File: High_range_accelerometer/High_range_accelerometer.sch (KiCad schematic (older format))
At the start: 55 parts, among them J1 USB_B_Micro, P1 KRC_PSoCWriter, U1 KRC_Conn_CAN, U2 NCP718ASN330T1G, U3 NCP718ASN500T1G, U4 NCV7342, U5 CY8C5868LTI-LP039, U6 H3LIS331DLTR, U7 W25N01GVxxIG-IT, Y2 Crystal_MHz

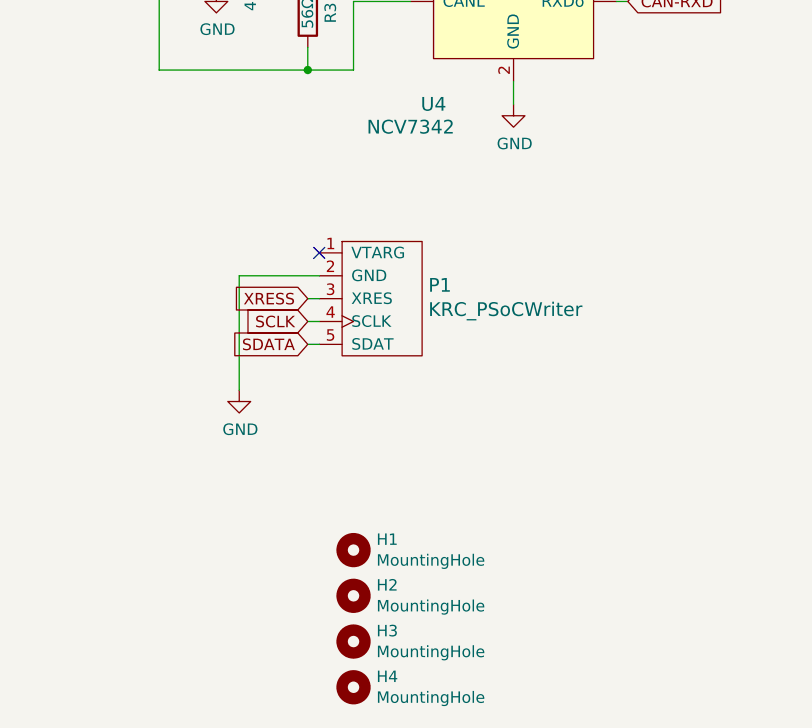
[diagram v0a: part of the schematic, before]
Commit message: add SVG and PDF and Gerber files
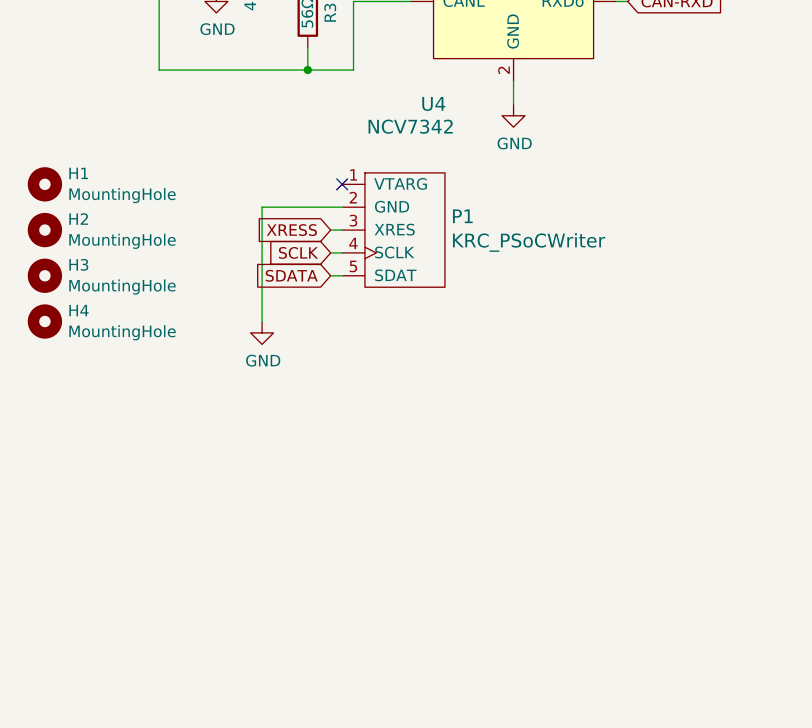
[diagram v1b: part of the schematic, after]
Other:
- moved on the sheet: H1, H2, H3, H4, P1
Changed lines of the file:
@@
 L High_range_accelerometer-rescue:KRC_PSoCWriter-KUT_Connector P1
 U 1 1 5D89CA7D
-P 2100 5500
-F 0 "P1" H 2377 5558 60  0000 L CNN
-F 1 "KRC_PSoCWriter" H 2377 5452 60  0000 L CNN
-F 2 "KUTKiCad_footprint:JST_JQ_05JQ-BT_1x05_P2.5mm_Vertical" H 2325 5500 60  0001 C CNN
-F 3 "" H 2325 5500 60  0000 C CNN
-	1    2100 5500
+P 2200 5200
+F 0 "P1" H 2477 5258 60  0000 L CNN
+F 1 "KRC_PSoCWriter" H 2477 5152 60  0000 L CNN
+F 2 "KUTKiCad_footprint:JST_JQ_05JQ-BT_1x05_P2.5mm_Vertical" H 2425 5200 60  0001 C CNN
+F 3 "" H 2425 5200 60  0000 C CNN
+	1    2200 5200
 	1    0    0    -1
 $EndComp
@@
 L power:GND #PWR03
 U 1 1 5D8A2416
-P 1550 5900
-F 0 "#PWR03" H 1550 5650 50  0001 C CNN
-F 1 "GND" H 1555 5727 50  0000 C CNN
-F 2 "" H 1550 5900 50  0001 C CNN
-F 3 "" H 1550 5900 50  0001 C CNN
-	1    1550 5900
-	1    0    0    -1
-$EndComp
-Wire Wire Line
-	1550 5900 1550 5400
-Wire Wire Line
-	1550 5400 1900 5400
-Text GLabel 1850 5500 0    50   Input ~ 0
+P 1650 5600
+F 0 "#PWR03" H 1650 5350 50  0001 C CNN
+F 1 "GND" H 1655 5427 50  0000 C CNN
+F 2 "" H 1650 5600 50  0001 C CNN
+F 3 "" H 1650 5600 50  0001 C CNN
+	1    1650 5600
+	1    0    0    -1
+$EndComp
+Wire Wire Line
+	1650 5600 1650 5100
+Wire Wire Line
+	1650 5100 2000 5100
+Text GLabel 1950 5200 0    50   Input ~ 0
 XRESS
-Text GLabel 1850 5600 0    50   Input ~ 0
+Text GLabel 1950 5300 0    50   Input ~ 0
 SCLK
-Text GLabel 1850 5700 0    50   Input ~ 0
+Text GLabel 1950 5400 0    50   Input ~ 0
 SDATA
 Wire Wire Line
-	1850 5700 1900 5700
-Wire Wire Line
-	1900 5600 1850 5600
-Wire Wire Line
-	1850 5500 1900 5500
+	1950 5400 2000 5400
+Wire Wire Line
+	2000 5300 1950 5300
+Wire Wire Line
+	1950 5200 2000 5200
 Text GLabel 4550 4150 0    50   Input ~ 0
 XRESS
@@
 Wire Wire Line
 	3250 4200 3200 4200
-NoConn ~ 1900 5300
+NoConn ~ 2000 5000
 $Comp
 L Device:Crystal Y2
@@
 L Mechanical:MountingHole H1
 U 1 1 5D9A09FB
-P 2050 6600
-F 0 "H1" H 2150 6646 50  0000 L CNN
-F 1 "MountingHole" H 2150 6555 50  0000 L CNN
-F 2 "MountingHole:MountingHole_3.2mm_M3" H 2050 6600 50  0001 C CNN
-F 3 "~" H 2050 6600 50  0001 C CNN
-	1    2050 6600
+P 700 5000
+F 0 "H1" H 800 5046 50  0000 L CNN
+F 1 "MountingHole" H 800 4955 50  0000 L CNN
+F 2 "MountingHole:MountingHole_3.2mm_M3" H 700 5000 50  0001 C CNN
+F 3 "~" H 700 5000 50  0001 C CNN
+	1    700  5000
 	1    0    0    -1
 $EndComp
@@
 L Mechanical:MountingHole H2
 U 1 1 5D9A0A93
-P 2050 6800
-F 0 "H2" H 2150 6846 50  0000 L CNN
-F 1 "MountingHole" H 2150 6755 50  0000 L CNN
-F 2 "MountingHole:MountingHole_3.2mm_M3" H 2050 6800 50  0001 C CNN
-F 3 "~" H 2050 6800 50  0001 C CNN
-	1    2050 6800
+P 700 5200
+F 0 "H2" H 800 5246 50  0000 L CNN
+F 1 "MountingHole" H 800 5155 50  0000 L CNN
+F 2 "MountingHole:MountingHole_3.2mm_M3" H 700 5200 50  0001 C CNN
+F 3 "~" H 700 5200 50  0001 C CNN
+	1    700  5200
 	1    0    0    -1
 $EndComp
@@
 L Mechanical:MountingHole H3
 U 1 1 5D9A0B13
-P 2050 7000
-F 0 "H3" H 2150 7046 50  0000 L CNN
-F 1 "MountingHole" H 2150 6955 50  0000 L CNN
-F 2 "MountingHole:MountingHole_3.2mm_M3" H 2050 7000 50  0001 C CNN
-F 3 "~" H 2050 7000 50  0001 C CNN
-	1    2050 7000
+P 700 5400
+F 0 "H3" H 800 5446 50  0000 L CNN
+F 1 "MountingHole" H 800 5355 50  0000 L CNN
+F 2 "MountingHole:MountingHole_3.2mm_M3" H 700 5400 50  0001 C CNN
+F 3 "~" H 700 5400 50  0001 C CNN
+	1    700  5400
 	1    0    0    -1
 $EndComp
@@
 L Mechanical:MountingHole H4
 U 1 1 5D9A0B95
-P 2050 7200
-F 0 "H4" H 2150 7246 50  0000 L CNN
-F 1 "MountingHole" H 2150 7155 50  0000 L CNN
-F 2 "MountingHole:MountingHole_3.2mm_M3" H 2050 7200 50  0001 C CNN
-F 3 "~" H 2050 7200 50  0001 C CNN
-	1    2050 7200
-	1    0    0    -1
-$EndComp
+P 700 5600
+F 0 "H4" H 800 5646 50  0000 L CNN
+F 1 "MountingHole" H 800 5555 50  0000 L CNN
+F 2 "MountingHole:MountingHole_3.2mm_M3" H 700 5600 50  0001 C CNN
+F 3 "~" H 700 5600 50  0001 C CNN
+	1    700  5600
+	1    0    0    -1
+$EndComp
